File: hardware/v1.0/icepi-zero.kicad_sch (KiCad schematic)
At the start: 25 parts, among them J1 Conn_02x20_Counter_Clockwise, SW1 SW_Push, U1 ECP5U_12_CABGA256

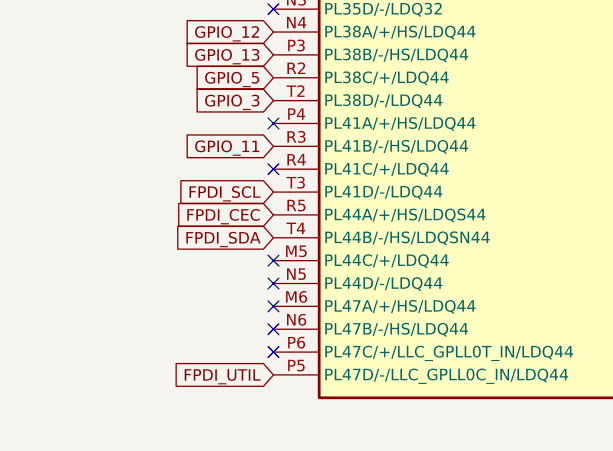
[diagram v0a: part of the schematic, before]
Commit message: Forgot to commit yesterday
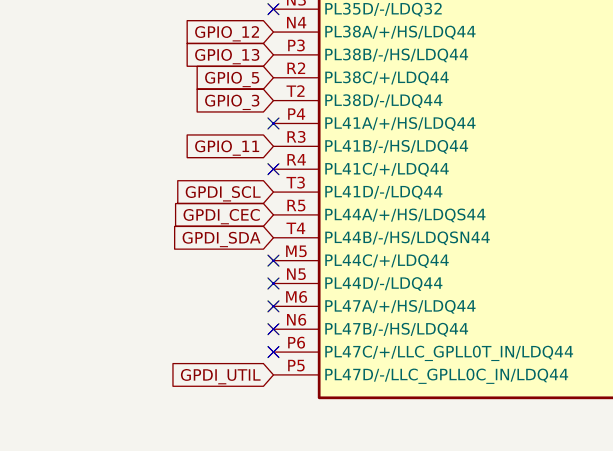
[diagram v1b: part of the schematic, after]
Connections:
- net FPDI_CEC renamed GPDI_CEC
- net FPDI_SCL renamed GPDI_SCL
- net FPDI_SDA renamed GPDI_SDA
- net FPDI_UTIL renamed GPDI_UTIL
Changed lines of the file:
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@@
 		)
 	)
-	(global_label "FPDI_SDA"
+	(global_label "GPDI_SDA"
 		(shape input)
 		(at 49.53 163.83 180)
@@
 		)
 	)
-	(global_label "FPDI_CEC"
+	(global_label "GPDI_CEC"
 		(shape input)
 		(at 49.53 161.29 180)
@@
 		)
 	)
-	(global_label "FPDI_UTIL"
+	(global_label "GPDI_UTIL"
 		(shape input)
 		(at 49.53 179.07 180)
@@
 		)
 	)
-	(global_label "FPDI_SCL"
+	(global_label "GPDI_SCL"
 		(shape input)
 		(at 49.53 158.75 180)
